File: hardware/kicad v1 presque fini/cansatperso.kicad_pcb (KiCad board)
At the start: 6 copper layers, 24.9 x 21.4 mm, 108 parts, among them IC1 2536030320001, IC2 LDO40LPU33RY, IC3 L7981TR, IC4 TSC102IDT, IC5 LDO40LPU33RY, J2 47309-2651, J3 connecteur gps, J4 connecteur radio, SW1 RSTBTN, SW2 boot, U1 STM32G431CBUx, U2 USBLC6-2SC6, Y1 Crystal_GND24_Small

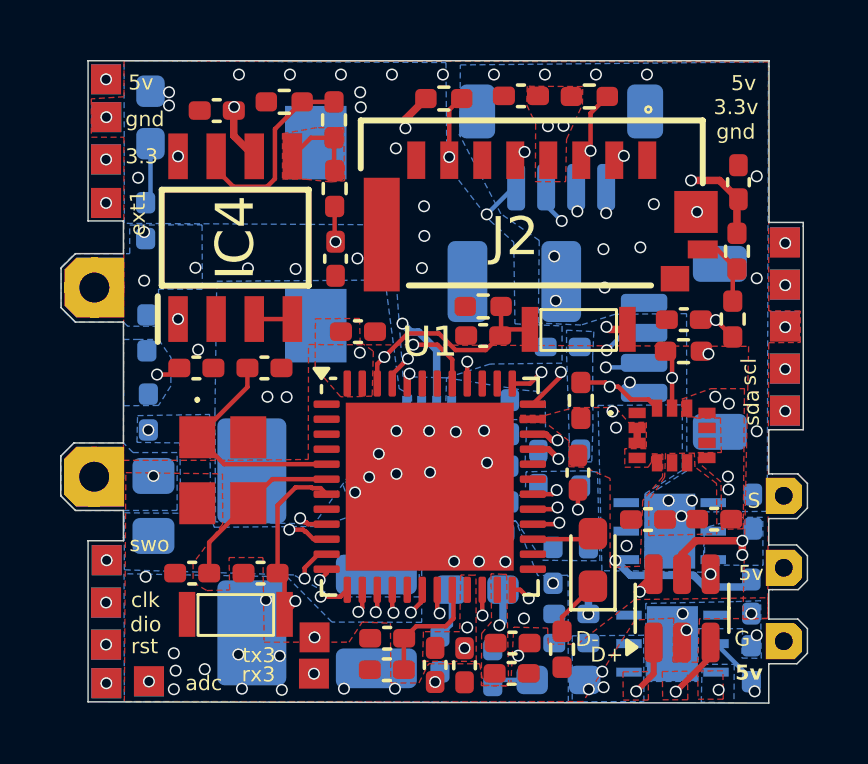
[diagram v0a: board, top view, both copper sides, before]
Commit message: finis
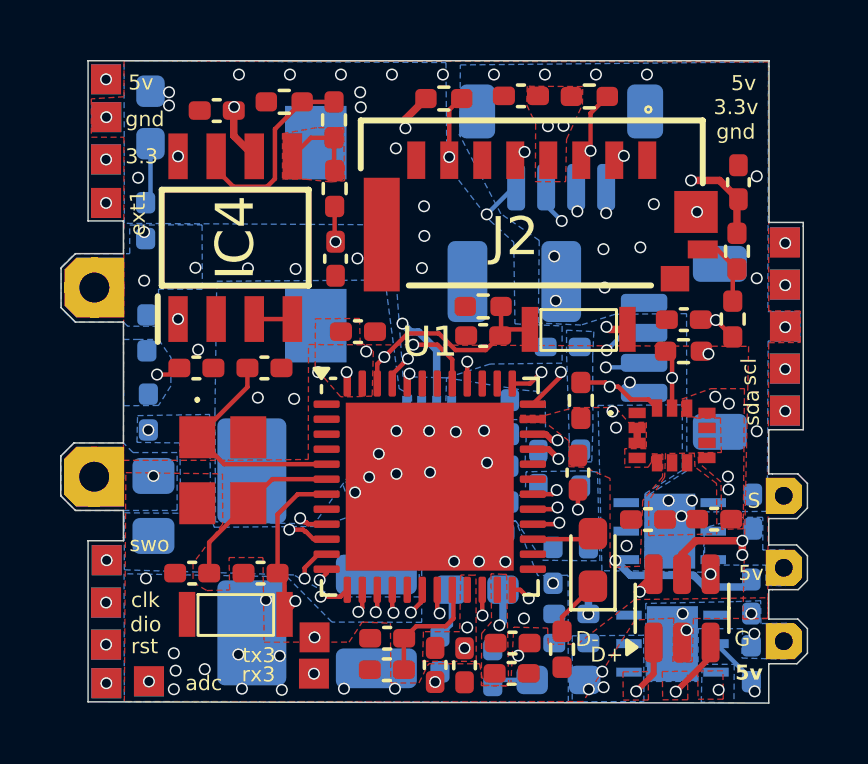
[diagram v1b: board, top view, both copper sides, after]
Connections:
- J3 pad MP: (no net) -> GND
- J4 pad : (no net) -> GND
- J4 pad MP: (no net) -> GND
- REF**1 pad 5v: (no net) -> +5V
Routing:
- net +3.3V: vias 20 -> 22
